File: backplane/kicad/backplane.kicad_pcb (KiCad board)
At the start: 4 copper layers, 141.2 x 81.1 mm, 6 parts, among them J1 weactstm32h7xx, J2 pcie_98, J3 pcie_98, J4 pcie_98, J5 pcie_98, J6 pcie_98

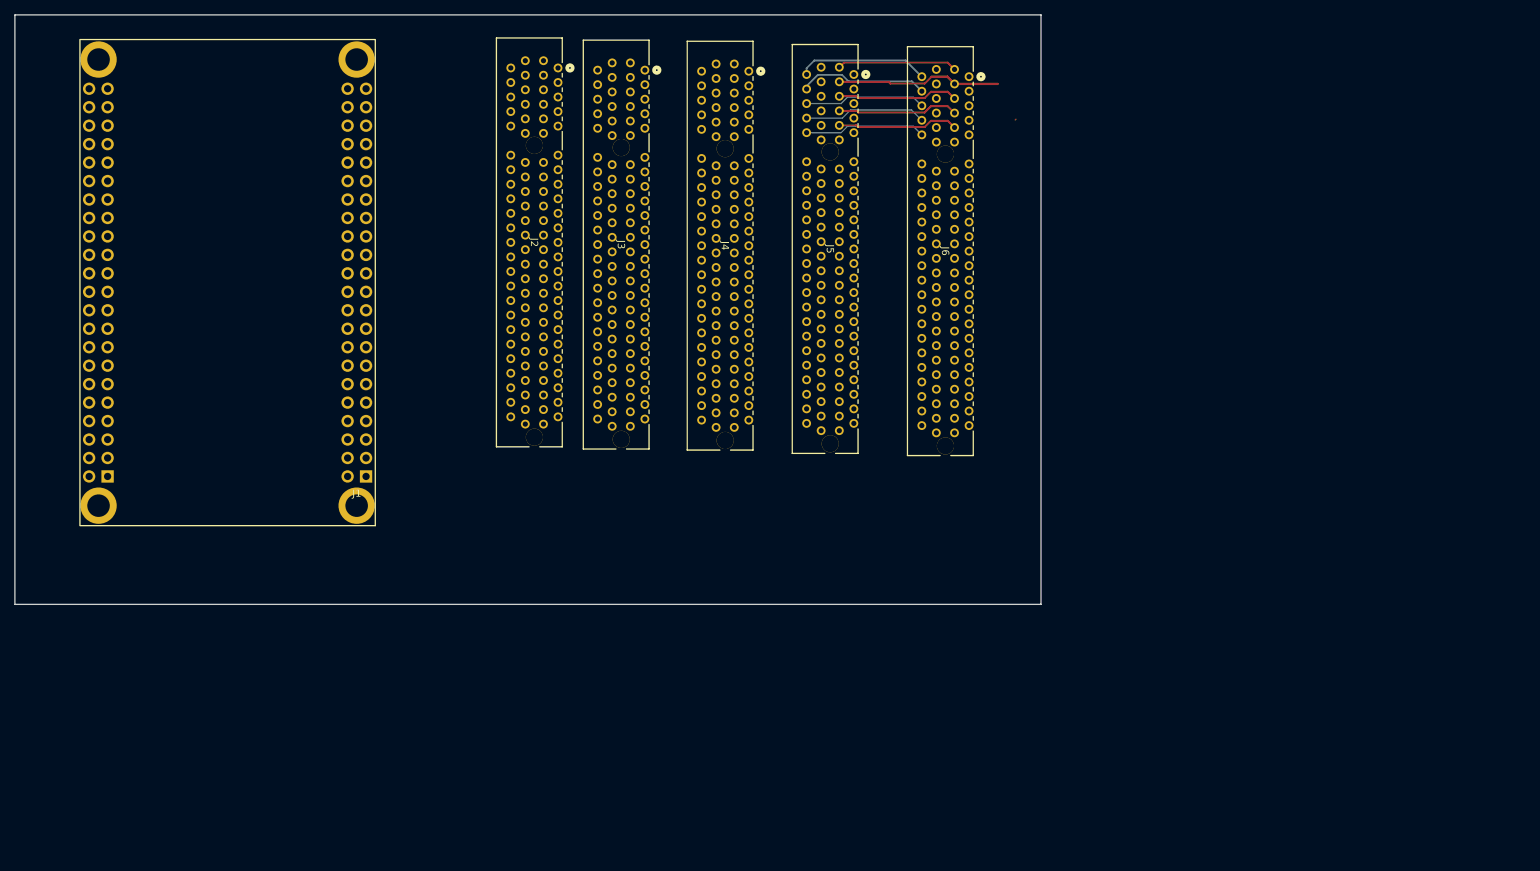
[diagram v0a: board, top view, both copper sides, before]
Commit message: Work in progress. Backlane kicad.
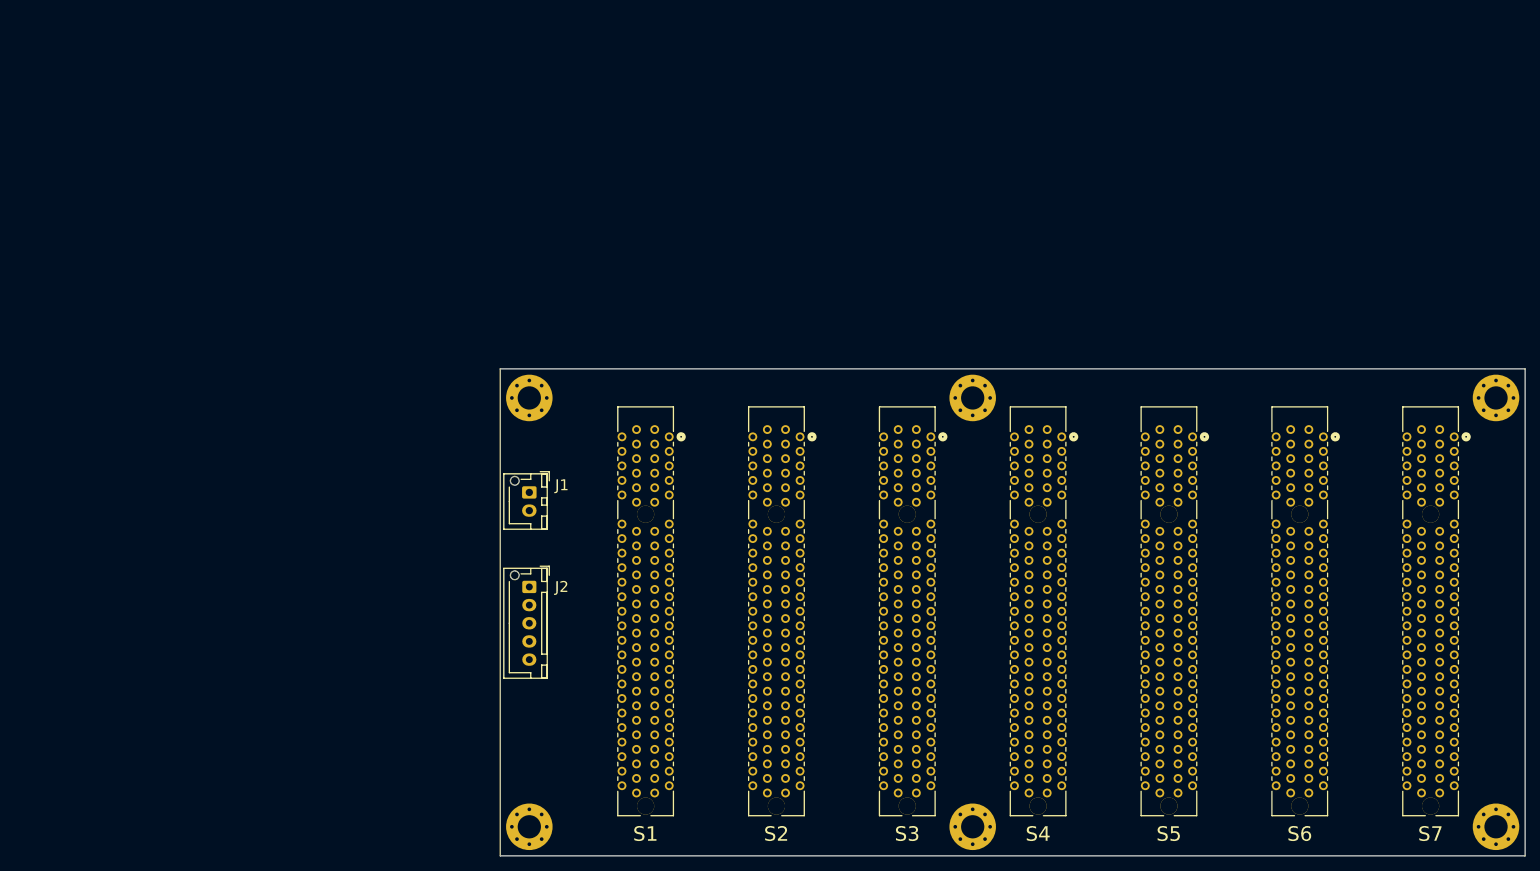
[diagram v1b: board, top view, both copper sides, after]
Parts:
- added H1: MountingHole, MountingHole:MountingHole_3.2mm_M3_Pad_Via, F.Cu at (84.0, 74.0)
- added H2: MountingHole, MountingHole:MountingHole_3.2mm_M3_Pad_Via, F.Cu at (145.0, 133.0)
- added H3: MountingHole, MountingHole:MountingHole_3.2mm_M3_Pad_Via, F.Cu at (84.0, 133.0)
- added H4: MountingHole, MountingHole:MountingHole_3.2mm_M3_Pad_Via, F.Cu at (217.0, 74.0)
- added H5: MountingHole, MountingHole:MountingHole_3.2mm_M3_Pad_Via, F.Cu at (145.0, 74.0)
- added H6: MountingHole, MountingHole:MountingHole_3.2mm_M3_Pad_Via, F.Cu at (217.0, 133.0)
- added J2: Conn_01x05_Pin, backplane:JST_XH_B5B-XH-AM_1x05_P2.50mm_Vertical, F.Cu at (84.0, 100.0)
- added S1: pcie_98, backplane:pcie_98_socket, F.Cu at (100.0, 90.0)
- added S7: pcie_98, backplane:pcie_98_socket, F.Cu at (208.0, 90.0)
- J1: value weactstm32h7xx -> Conn_01x02_Pin; footprint main_board:weact_stm32fh750 -> backplane:JST_XH_B2B-XH-AM_1x02_P2.50mm_Vertical
- S2: renamed from J2; footprint main_board:pcie_98_socket -> backplane:pcie_98_socket
- S3: renamed from J3; footprint main_board:pcie_98_socket -> backplane:pcie_98_socket
- S4: renamed from J4; footprint main_board:pcie_98_socket -> backplane:pcie_98_socket
- S5: renamed from J5; footprint main_board:pcie_98_socket -> backplane:pcie_98_socket
- S6: renamed from J6; footprint main_board:pcie_98_socket -> backplane:pcie_98_socket
- moved S6 77.5 mm to (190.0, 90.0)
- moved S5 76.4 mm to (172.0, 90.0)
- moved S4 74.7 mm to (154.0, 90.0)
- moved S3 72.9 mm to (136.0, 90.0)
- moved S2 70.1 mm to (118.0, 90.0)
- moved J1 50.6 mm to (84.0, 87.0), turned to -90 degrees
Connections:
- J1 pad 1: /GND -> unconnected-(J1-Pin_1-Pad1)
- J1 pad 2: /5V -> unconnected-(J1-Pin_2-Pad2)
- S2 pad A1: unconnected-(J2-Pin_a1-PadA1) -> /A1
- S2 pad A10: unconnected-(J2-Pin_a10-PadA10) -> /A10
- S2 pad A11: unconnected-(J2-Pin_A11-PadA11) -> /A11
- S2 pad A12: unconnected-(J2-Pin_a12-PadA12) -> /A12
- S2 pad A13: unconnected-(J2-Pin_a13-PadA13) -> /A13
- S2 pad A14: unconnected-(J2-Pin_a14-PadA14) -> /A14
- S2 pad A15: unconnected-(J2-Pin_a15-PadA15) -> /A15
- S2 pad A16: unconnected-(J2-Pin_a16-PadA16) -> /A16
- S2 pad A17: unconnected-(J2-Pin_a17-PadA17) -> /A17
- S2 pad A18: unconnected-(J2-Pin_a18-PadA18) -> /A18
- S2 pad A19: unconnected-(J2-Pin_a19-PadA19) -> /A19
- S2 pad A2: unconnected-(J2-Pin_a2-PadA2) -> /A2
- S2 pad A21: unconnected-(J2-Pin_a21-PadA21) -> /A21
- S2 pad A22: unconnected-(J2-Pin_a22-PadA22) -> /A22
- S2 pad A23: unconnected-(J2-Pin_a23-PadA23) -> /A23
- S2 pad A24: unconnected-(J2-Pin_a24-PadA24) -> /A24
- S2 pad A25: unconnected-(J2-Pin_a25-PadA25) -> /A25
- S2 pad A26: unconnected-(J2-Pin_a26-PadA26) -> /A26
- S2 pad A27: unconnected-(J2-Pin_a27-PadA27) -> /A27
- S2 pad A28: unconnected-(J2-Pin_a28-PadA28) -> /A28
- S2 pad A29: unconnected-(J2-Pin_a29-PadA29) -> /A29
- S2 pad A3: unconnected-(J2-Pin_a3-PadA3) -> /A3
- S2 pad A30: unconnected-(J2-Pin_a30-PadA30) -> /A30
- S2 pad A31: unconnected-(J2-Pin_a31-PadA31) -> /A31
- S2 pad A32: unconnected-(J2-Pin_a32-PadA32) -> /A32
- S2 pad A33: unconnected-(J2-Pin_a33-PadA33) -> /A33
- S2 pad A34: unconnected-(J2-Pin_a34-PadA34) -> /A34
- S2 pad A35: unconnected-(J2-Pin_a35-PadA35) -> /A35
- S2 pad A36: unconnected-(J2-Pin_a36-PadA36) -> /A36
- S2 pad A37: unconnected-(J2-Pin_a37-PadA37) -> /A37
- S2 pad A38: unconnected-(J2-Pin_a38-PadA38) -> /A38
- S2 pad A39: unconnected-(J2-Pin_a39-PadA39) -> /A39
- S2 pad A4: unconnected-(J2-Pin_a4-PadA4) -> /A4
- S2 pad A40: unconnected-(J2-Pin_a40-PadA40) -> /A40
- S2 pad A41: unconnected-(J2-Pin_a41-PadA41) -> /A41
- S2 pad A42: unconnected-(J2-Pin_a42-PadA42) -> /A42
- S2 pad A43: unconnected-(J2-Pin_a43-PadA43) -> /A43
- S2 pad A44: unconnected-(J2-Pin_a44-PadA44) -> /A44
- S2 pad A45: unconnected-(J2-Pin_a45-PadA45) -> /A45
- S2 pad A46: unconnected-(J2-Pin_a46-PadA46) -> /A46
- S2 pad A47: unconnected-(J2-Pin_a47-PadA47) -> /A47
- S2 pad A48: unconnected-(J2-Pin_a48-PadA48) -> /A48
- S2 pad A49: unconnected-(J2-Pin_a49-PadA49) -> /A49
- S2 pad A5: unconnected-(J2-Pin_a5-PadA5) -> /A5
- S2 pad A6: unconnected-(J2-Pin_a6-PadA6) -> /A6
- S2 pad A7: unconnected-(J2-Pin_a7-PadA7) -> /A7
- S2 pad A8: unconnected-(J2-Pin_a8-PadA8) -> /A8
- S2 pad A9: unconnected-(J2-Pin_a9-PadA9) -> /A9
- S2 pad B1: unconnected-(J2-Pin_b1-PadB1) -> /B1
- S2 pad B10: unconnected-(J2-Pin_b10-PadB10) -> /B10
- S2 pad B11: unconnected-(J2-Pin_b11-PadB11) -> /B11
- S2 pad B12: unconnected-(J2-Pin_b12-PadB12) -> /B12
- S2 pad B13: unconnected-(J2-Pin_b13-PadB13) -> /B13
- S2 pad B14: unconnected-(J2-Pin_b14-PadB14) -> /B14
- S2 pad B15: unconnected-(J2-Pin_b15-PadB15) -> /B15
- S2 pad B16: unconnected-(J2-Pin_b16-PadB16) -> /B16
- S2 pad B17: unconnected-(J2-Pin_b17-PadB17) -> /B17
- S2 pad B18: unconnected-(J2-Pin_b18-PadB18) -> /B18
- S2 pad B19: unconnected-(J2-Pin_b19-PadB19) -> /B19
- S2 pad B2: unconnected-(J2-Pin_b2-PadB2) -> /B2
- S2 pad B20: unconnected-(J2-Pin_b20-PadB20) -> /B20
- S2 pad B21: unconnected-(J2-Pin_b21-PadB21) -> /B21
- S2 pad B22: unconnected-(J2-Pin_b22-PadB22) -> /B22
- S2 pad B23: unconnected-(J2-Pin_b23-PadB23) -> /B23
- S2 pad B3: unconnected-(J2-Pin_b3-PadB3) -> /B3
- S2 pad B4: unconnected-(J2-Pin_b4-PadB4) -> /B4
- S2 pad B5: unconnected-(J2-Pin_b5-PadB5) -> /B5
- S2 pad B6: unconnected-(J2-Pin_b6-PadB6) -> /B6
- S2 pad B7: unconnected-(J2-Pin_b7-PadB7) -> /B7
- S2 pad B8: unconnected-(J2-Pin_b8-PadB8) -> /B8
- S2 pad B9: unconnected-(J2-Pin_b9-PadB9) -> /B9
- S3 pad A1: unconnected-(J3-Pin_a1-PadA1) -> /A1
- S3 pad A10: unconnected-(J3-Pin_a10-PadA10) -> /A10
- S3 pad A11: unconnected-(J3-Pin_A11-PadA11) -> /A11
- S3 pad A12: unconnected-(J3-Pin_a12-PadA12) -> /A12
- S3 pad A13: unconnected-(J3-Pin_a13-PadA13) -> /A13
- S3 pad A14: unconnected-(J3-Pin_a14-PadA14) -> /A14
- S3 pad A15: unconnected-(J3-Pin_a15-PadA15) -> /A15
- S3 pad A16: unconnected-(J3-Pin_a16-PadA16) -> /A16
- S3 pad A17: unconnected-(J3-Pin_a17-PadA17) -> /A17
- S3 pad A18: unconnected-(J3-Pin_a18-PadA18) -> /A18
- S3 pad A19: unconnected-(J3-Pin_a19-PadA19) -> /A19
- S3 pad A2: unconnected-(J3-Pin_a2-PadA2) -> /A2
- S3 pad A21: unconnected-(J3-Pin_a21-PadA21) -> /A21
- S3 pad A22: unconnected-(J3-Pin_a22-PadA22) -> /A22
- S3 pad A23: unconnected-(J3-Pin_a23-PadA23) -> /A23
- S3 pad A24: unconnected-(J3-Pin_a24-PadA24) -> /A24
- S3 pad A25: unconnected-(J3-Pin_a25-PadA25) -> /A25
- S3 pad A26: unconnected-(J3-Pin_a26-PadA26) -> /A26
- S3 pad A27: unconnected-(J3-Pin_a27-PadA27) -> /A27
- S3 pad A28: unconnected-(J3-Pin_a28-PadA28) -> /A28
- S3 pad A29: unconnected-(J3-Pin_a29-PadA29) -> /A29
- S3 pad A3: unconnected-(J3-Pin_a3-PadA3) -> /A3
- S3 pad A30: unconnected-(J3-Pin_a30-PadA30) -> /A30
- S3 pad A31: unconnected-(J3-Pin_a31-PadA31) -> /A31
- S3 pad A32: unconnected-(J3-Pin_a32-PadA32) -> /A32
- S3 pad A33: unconnected-(J3-Pin_a33-PadA33) -> /A33
- S3 pad A34: unconnected-(J3-Pin_a34-PadA34) -> /A34
- S3 pad A35: unconnected-(J3-Pin_a35-PadA35) -> /A35
- S3 pad A36: unconnected-(J3-Pin_a36-PadA36) -> /A36
- S3 pad A37: unconnected-(J3-Pin_a37-PadA37) -> /A37
- S3 pad A38: unconnected-(J3-Pin_a38-PadA38) -> /A38
- S3 pad A39: unconnected-(J3-Pin_a39-PadA39) -> /A39
- S3 pad A4: unconnected-(J3-Pin_a4-PadA4) -> /A4
- S3 pad A40: unconnected-(J3-Pin_a40-PadA40) -> /A40
- S3 pad A41: unconnected-(J3-Pin_a41-PadA41) -> /A41
- S3 pad A42: unconnected-(J3-Pin_a42-PadA42) -> /A42
- S3 pad A43: unconnected-(J3-Pin_a43-PadA43) -> /A43
- S3 pad A44: unconnected-(J3-Pin_a44-PadA44) -> /A44
- S3 pad A45: unconnected-(J3-Pin_a45-PadA45) -> /A45
- S3 pad A46: unconnected-(J3-Pin_a46-PadA46) -> /A46
- S3 pad A47: unconnected-(J3-Pin_a47-PadA47) -> /A47
- S3 pad A48: unconnected-(J3-Pin_a48-PadA48) -> /A48
- S3 pad A49: unconnected-(J3-Pin_a49-PadA49) -> /A49
- S3 pad A5: unconnected-(J3-Pin_a5-PadA5) -> /A5
- S3 pad A6: unconnected-(J3-Pin_a6-PadA6) -> /A6
- S3 pad A7: unconnected-(J3-Pin_a7-PadA7) -> /A7
- S3 pad A8: unconnected-(J3-Pin_a8-PadA8) -> /A8
- S3 pad A9: unconnected-(J3-Pin_a9-PadA9) -> /A9
- S3 pad B1: unconnected-(J3-Pin_b1-PadB1) -> /B1
- S3 pad B10: unconnected-(J3-Pin_b10-PadB10) -> /B10
- S3 pad B11: unconnected-(J3-Pin_b11-PadB11) -> /B11
- S3 pad B12: unconnected-(J3-Pin_b12-PadB12) -> /B12
- S3 pad B13: unconnected-(J3-Pin_b13-PadB13) -> /B13
- S3 pad B14: unconnected-(J3-Pin_b14-PadB14) -> /B14
- S3 pad B15: unconnected-(J3-Pin_b15-PadB15) -> /B15
- S3 pad B16: unconnected-(J3-Pin_b16-PadB16) -> /B16
- S3 pad B17: unconnected-(J3-Pin_b17-PadB17) -> /B17
- S3 pad B18: unconnected-(J3-Pin_b18-PadB18) -> /B18
- S3 pad B19: unconnected-(J3-Pin_b19-PadB19) -> /B19
- S3 pad B2: unconnected-(J3-Pin_b2-PadB2) -> /B2
- S3 pad B20: unconnected-(J3-Pin_b20-PadB20) -> /B20
- S3 pad B21: unconnected-(J3-Pin_b21-PadB21) -> /B21
- S3 pad B22: unconnected-(J3-Pin_b22-PadB22) -> /B22
- S3 pad B23: unconnected-(J3-Pin_b23-PadB23) -> /B23
- S3 pad B3: unconnected-(J3-Pin_b3-PadB3) -> /B3
- S3 pad B4: unconnected-(J3-Pin_b4-PadB4) -> /B4
- S3 pad B5: unconnected-(J3-Pin_b5-PadB5) -> /B5
- S3 pad B6: unconnected-(J3-Pin_b6-PadB6) -> /B6
- S3 pad B7: unconnected-(J3-Pin_b7-PadB7) -> /B7
- S3 pad B8: unconnected-(J3-Pin_b8-PadB8) -> /B8
- S3 pad B9: unconnected-(J3-Pin_b9-PadB9) -> /B9
- S4 pad A1: unconnected-(J4-Pin_a1-PadA1) -> /A1
- S4 pad A10: unconnected-(J4-Pin_a10-PadA10) -> /A10
- S4 pad A11: unconnected-(J4-Pin_A11-PadA11) -> /A11
- S4 pad A12: unconnected-(J4-Pin_a12-PadA12) -> /A12
- S4 pad A13: unconnected-(J4-Pin_a13-PadA13) -> /A13
- S4 pad A14: unconnected-(J4-Pin_a14-PadA14) -> /A14
- S4 pad A15: unconnected-(J4-Pin_a15-PadA15) -> /A15
- S4 pad A16: unconnected-(J4-Pin_a16-PadA16) -> /A16
- S4 pad A17: unconnected-(J4-Pin_a17-PadA17) -> /A17
- S4 pad A18: unconnected-(J4-Pin_a18-PadA18) -> /A18
- S4 pad A19: unconnected-(J4-Pin_a19-PadA19) -> /A19
- S4 pad A2: unconnected-(J4-Pin_a2-PadA2) -> /A2
- S4 pad A21: unconnected-(J4-Pin_a21-PadA21) -> /A21
- S4 pad A22: unconnected-(J4-Pin_a22-PadA22) -> /A22
- S4 pad A23: unconnected-(J4-Pin_a23-PadA23) -> /A23
- S4 pad A24: unconnected-(J4-Pin_a24-PadA24) -> /A24
- S4 pad A25: unconnected-(J4-Pin_a25-PadA25) -> /A25
- S4 pad A26: unconnected-(J4-Pin_a26-PadA26) -> /A26
- S4 pad A27: unconnected-(J4-Pin_a27-PadA27) -> /A27
- S4 pad A28: unconnected-(J4-Pin_a28-PadA28) -> /A28
- S4 pad A29: unconnected-(J4-Pin_a29-PadA29) -> /A29
- S4 pad A3: unconnected-(J4-Pin_a3-PadA3) -> /A3
- S4 pad A30: unconnected-(J4-Pin_a30-PadA30) -> /A30
- S4 pad A31: unconnected-(J4-Pin_a31-PadA31) -> /A31
- S4 pad A32: unconnected-(J4-Pin_a32-PadA32) -> /A32
- S4 pad A33: unconnected-(J4-Pin_a33-PadA33) -> /A33
- S4 pad A34: unconnected-(J4-Pin_a34-PadA34) -> /A34
- S4 pad A35: unconnected-(J4-Pin_a35-PadA35) -> /A35
- S4 pad A36: unconnected-(J4-Pin_a36-PadA36) -> /A36
- S4 pad A37: unconnected-(J4-Pin_a37-PadA37) -> /A37
- S4 pad A38: unconnected-(J4-Pin_a38-PadA38) -> /A38
- S4 pad A39: unconnected-(J4-Pin_a39-PadA39) -> /A39
- S4 pad A4: unconnected-(J4-Pin_a4-PadA4) -> /A4
- S4 pad A40: unconnected-(J4-Pin_a40-PadA40) -> /A40
- S4 pad A41: unconnected-(J4-Pin_a41-PadA41) -> /A41
- S4 pad A42: unconnected-(J4-Pin_a42-PadA42) -> /A42
- S4 pad A43: unconnected-(J4-Pin_a43-PadA43) -> /A43
- S4 pad A44: unconnected-(J4-Pin_a44-PadA44) -> /A44
- S4 pad A45: unconnected-(J4-Pin_a45-PadA45) -> /A45
- S4 pad A46: unconnected-(J4-Pin_a46-PadA46) -> /A46
- S4 pad A47: unconnected-(J4-Pin_a47-PadA47) -> /A47
- S4 pad A48: unconnected-(J4-Pin_a48-PadA48) -> /A48
- S4 pad A49: unconnected-(J4-Pin_a49-PadA49) -> /A49
- S4 pad A5: unconnected-(J4-Pin_a5-PadA5) -> /A5
- S4 pad A6: unconnected-(J4-Pin_a6-PadA6) -> /A6
- S4 pad A7: unconnected-(J4-Pin_a7-PadA7) -> /A7
- S4 pad A8: unconnected-(J4-Pin_a8-PadA8) -> /A8
- S4 pad A9: unconnected-(J4-Pin_a9-PadA9) -> /A9
- S4 pad B1: unconnected-(J4-Pin_b1-PadB1) -> /B1
- S4 pad B10: unconnected-(J4-Pin_b10-PadB10) -> /B10
- S4 pad B11: unconnected-(J4-Pin_b11-PadB11) -> /B11
- S4 pad B12: unconnected-(J4-Pin_b12-PadB12) -> /B12
- S4 pad B13: unconnected-(J4-Pin_b13-PadB13) -> /B13
- S4 pad B14: unconnected-(J4-Pin_b14-PadB14) -> /B14
- S4 pad B15: unconnected-(J4-Pin_b15-PadB15) -> /B15
- S4 pad B16: unconnected-(J4-Pin_b16-PadB16) -> /B16
- S4 pad B17: unconnected-(J4-Pin_b17-PadB17) -> /B17
- S4 pad B18: unconnected-(J4-Pin_b18-PadB18) -> /B18
- S4 pad B19: unconnected-(J4-Pin_b19-PadB19) -> /B19
- S4 pad B2: unconnected-(J4-Pin_b2-PadB2) -> /B2
- S4 pad B20: unconnected-(J4-Pin_b20-PadB20) -> /B20
- S4 pad B21: unconnected-(J4-Pin_b21-PadB21) -> /B21
- S4 pad B22: unconnected-(J4-Pin_b22-PadB22) -> /B22
- S4 pad B23: unconnected-(J4-Pin_b23-PadB23) -> /B23
- S4 pad B3: unconnected-(J4-Pin_b3-PadB3) -> /B3
- S4 pad B4: unconnected-(J4-Pin_b4-PadB4) -> /B4
- S4 pad B5: unconnected-(J4-Pin_b5-PadB5) -> /B5
- S4 pad B6: unconnected-(J4-Pin_b6-PadB6) -> /B6
- S4 pad B7: unconnected-(J4-Pin_b7-PadB7) -> /B7
- S4 pad B8: unconnected-(J4-Pin_b8-PadB8) -> /B8
- S4 pad B9: unconnected-(J4-Pin_b9-PadB9) -> /B9
- S5 pad A12: unconnected-(J5-Pin_a12-PadA12) -> /A12
- S5 pad A13: unconnected-(J5-Pin_a13-PadA13) -> /A13
- S5 pad A14: unconnected-(J5-Pin_a14-PadA14) -> /A14
- S5 pad A15: unconnected-(J5-Pin_a15-PadA15) -> /A15
- S5 pad A16: unconnected-(J5-Pin_a16-PadA16) -> /A16
- S5 pad A17: unconnected-(J5-Pin_a17-PadA17) -> /A17
- S5 pad A18: unconnected-(J5-Pin_a18-PadA18) -> /A18
- S5 pad A19: unconnected-(J5-Pin_a19-PadA19) -> /A19
- S5 pad A21: unconnected-(J5-Pin_a21-PadA21) -> /A21
- S5 pad A22: unconnected-(J5-Pin_a22-PadA22) -> /A22
- S5 pad A23: unconnected-(J5-Pin_a23-PadA23) -> /A23
- S5 pad A24: unconnected-(J5-Pin_a24-PadA24) -> /A24
- S5 pad A25: unconnected-(J5-Pin_a25-PadA25) -> /A25
- S5 pad A26: unconnected-(J5-Pin_a26-PadA26) -> /A26
- S5 pad A27: unconnected-(J5-Pin_a27-PadA27) -> /A27
- S5 pad A28: unconnected-(J5-Pin_a28-PadA28) -> /A28
- S5 pad A29: unconnected-(J5-Pin_a29-PadA29) -> /A29
- S5 pad A30: unconnected-(J5-Pin_a30-PadA30) -> /A30
- S5 pad A31: unconnected-(J5-Pin_a31-PadA31) -> /A31
- S5 pad A32: unconnected-(J5-Pin_a32-PadA32) -> /A32
- S5 pad A33: unconnected-(J5-Pin_a33-PadA33) -> /A33
- S5 pad A34: unconnected-(J5-Pin_a34-PadA34) -> /A34
- S5 pad A35: unconnected-(J5-Pin_a35-PadA35) -> /A35
- S5 pad A36: unconnected-(J5-Pin_a36-PadA36) -> /A36
- S5 pad A37: unconnected-(J5-Pin_a37-PadA37) -> /A37
- S5 pad A38: unconnected-(J5-Pin_a38-PadA38) -> /A38
- S5 pad A39: unconnected-(J5-Pin_a39-PadA39) -> /A39
- S5 pad A40: unconnected-(J5-Pin_a40-PadA40) -> /A40
- S5 pad A41: unconnected-(J5-Pin_a41-PadA41) -> /A41
- S5 pad A42: unconnected-(J5-Pin_a42-PadA42) -> /A42
- S5 pad A43: unconnected-(J5-Pin_a43-PadA43) -> /A43
- S5 pad A44: unconnected-(J5-Pin_a44-PadA44) -> /A44
- S5 pad A45: unconnected-(J5-Pin_a45-PadA45) -> /A45
- S5 pad A46: unconnected-(J5-Pin_a46-PadA46) -> /A46
- S5 pad A47: unconnected-(J5-Pin_a47-PadA47) -> /A47
- S5 pad A48: unconnected-(J5-Pin_a48-PadA48) -> /A48
- S5 pad A49: unconnected-(J5-Pin_a49-PadA49) -> /A49
- S5 pad B12: unconnected-(J5-Pin_b12-PadB12) -> /B12
- S5 pad B13: unconnected-(J5-Pin_b13-PadB13) -> /B13
- S5 pad B14: unconnected-(J5-Pin_b14-PadB14) -> /B14
- S5 pad B15: unconnected-(J5-Pin_b15-PadB15) -> /B15
- S5 pad B16: unconnected-(J5-Pin_b16-PadB16) -> /B16
- S5 pad B17: unconnected-(J5-Pin_b17-PadB17) -> /B17
- S5 pad B18: unconnected-(J5-Pin_b18-PadB18) -> /B18
- S5 pad B19: unconnected-(J5-Pin_b19-PadB19) -> /B19
- S5 pad B20: unconnected-(J5-Pin_b20-PadB20) -> /B20
- S5 pad B21: unconnected-(J5-Pin_b21-PadB21) -> /B21
- S5 pad B22: unconnected-(J5-Pin_b22-PadB22) -> /B22
- S5 pad B23: unconnected-(J5-Pin_b23-PadB23) -> /B23
- S6 pad A12: unconnected-(J6-Pin_a12-PadA12) -> /A12
- S6 pad A13: unconnected-(J6-Pin_a13-PadA13) -> /A13
- S6 pad A14: unconnected-(J6-Pin_a14-PadA14) -> /A14
- S6 pad A15: unconnected-(J6-Pin_a15-PadA15) -> /A15
- S6 pad A16: unconnected-(J6-Pin_a16-PadA16) -> /A16
- S6 pad A17: unconnected-(J6-Pin_a17-PadA17) -> /A17
- S6 pad A18: unconnected-(J6-Pin_a18-PadA18) -> /A18
- S6 pad A19: unconnected-(J6-Pin_a19-PadA19) -> /A19
- S6 pad A21: unconnected-(J6-Pin_a21-PadA21) -> /A21
- S6 pad A22: unconnected-(J6-Pin_a22-PadA22) -> /A22
- S6 pad A23: unconnected-(J6-Pin_a23-PadA23) -> /A23
- S6 pad A24: unconnected-(J6-Pin_a24-PadA24) -> /A24
- S6 pad A25: unconnected-(J6-Pin_a25-PadA25) -> /A25
- S6 pad A26: unconnected-(J6-Pin_a26-PadA26) -> /A26
- S6 pad A27: unconnected-(J6-Pin_a27-PadA27) -> /A27
- S6 pad A28: unconnected-(J6-Pin_a28-PadA28) -> /A28
- S6 pad A29: unconnected-(J6-Pin_a29-PadA29) -> /A29
- S6 pad A30: unconnected-(J6-Pin_a30-PadA30) -> /A30
- S6 pad A31: unconnected-(J6-Pin_a31-PadA31) -> /A31
- S6 pad A32: unconnected-(J6-Pin_a32-PadA32) -> /A32
- S6 pad A33: unconnected-(J6-Pin_a33-PadA33) -> /A33
- S6 pad A34: unconnected-(J6-Pin_a34-PadA34) -> /A34
- S6 pad A35: unconnected-(J6-Pin_a35-PadA35) -> /A35
- S6 pad A36: unconnected-(J6-Pin_a36-PadA36) -> /A36
- S6 pad A37: unconnected-(J6-Pin_a37-PadA37) -> /A37
- S6 pad A38: unconnected-(J6-Pin_a38-PadA38) -> /A38
- S6 pad A39: unconnected-(J6-Pin_a39-PadA39) -> /A39
- S6 pad A40: unconnected-(J6-Pin_a40-PadA40) -> /A40
- S6 pad A41: unconnected-(J6-Pin_a41-PadA41) -> /A41
- S6 pad A42: unconnected-(J6-Pin_a42-PadA42) -> /A42
- S6 pad A43: unconnected-(J6-Pin_a43-PadA43) -> /A43
- S6 pad A44: unconnected-(J6-Pin_a44-PadA44) -> /A44
- S6 pad A45: unconnected-(J6-Pin_a45-PadA45) -> /A45
- S6 pad A46: unconnected-(J6-Pin_a46-PadA46) -> /A46
- S6 pad A47: unconnected-(J6-Pin_a47-PadA47) -> /A47
- S6 pad A48: unconnected-(J6-Pin_a48-PadA48) -> /A48
- S6 pad A49: unconnected-(J6-Pin_a49-PadA49) -> /A49
- S6 pad B12: unconnected-(J6-Pin_b12-PadB12) -> /B12
- S6 pad B13: unconnected-(J6-Pin_b13-PadB13) -> /B13
- S6 pad B14: unconnected-(J6-Pin_b14-PadB14) -> /B14
- S6 pad B15: unconnected-(J6-Pin_b15-PadB15) -> /B15
- S6 pad B16: unconnected-(J6-Pin_b16-PadB16) -> /B16
- S6 pad B17: unconnected-(J6-Pin_b17-PadB17) -> /B17
- S6 pad B18: unconnected-(J6-Pin_b18-PadB18) -> /B18
- S6 pad B19: unconnected-(J6-Pin_b19-PadB19) -> /B19
- S6 pad B20: unconnected-(J6-Pin_b20-PadB20) -> /B20
- S6 pad B21: unconnected-(J6-Pin_b21-PadB21) -> /B21
- S6 pad B22: unconnected-(J6-Pin_b22-PadB22) -> /B22
- S6 pad B23: unconnected-(J6-Pin_b23-PadB23) -> /B23
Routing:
- net /A3: track 22.7 -> 0.00 mm
- net /B2: track 18.1 -> 0.00 mm
- net /B4: track 17.8 -> 0.00 mm
- net /B3: track 17.6 -> 0.00 mm
- net /A8: track 17.6 -> 0.00 mm
- net /A2: track 17.5 -> 0.00 mm
- net /A6: track 17.5 -> 0.00 mm
- net /A10: track 17.4 -> 0.00 mm
- net /A4: track 17.4 -> 0.00 mm
- net /B8: track 16.9 -> 0.00 mm
- net /B11: track 16.8 -> 0.00 mm
- net /B9: track 16.7 -> 0.00 mm
- net /B7: track 16.7 -> 0.00 mm
- net /B5: track 16.7 -> 0.00 mm
- net /B1: track 16.7 -> 0.00 mm
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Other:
- board size 141.2 x 81.1 mm -> 141 x 67 mm
